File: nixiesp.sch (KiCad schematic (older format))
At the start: 50 parts, among them J1 Power 9-15V, J2 ESP8266, J3 Nixie PSU low, J4 CONN_01X02, Q1 BS107, Q2 BS107, Q3 BS107, Q4 BS107, U1 74HC595, U10 LM1117-3.3, U2 K155ID1, U3 K155ID1, U4 K155ID1, U5 74HC595, U6 K155ID1, U7 K155ID1, U8 74HC595

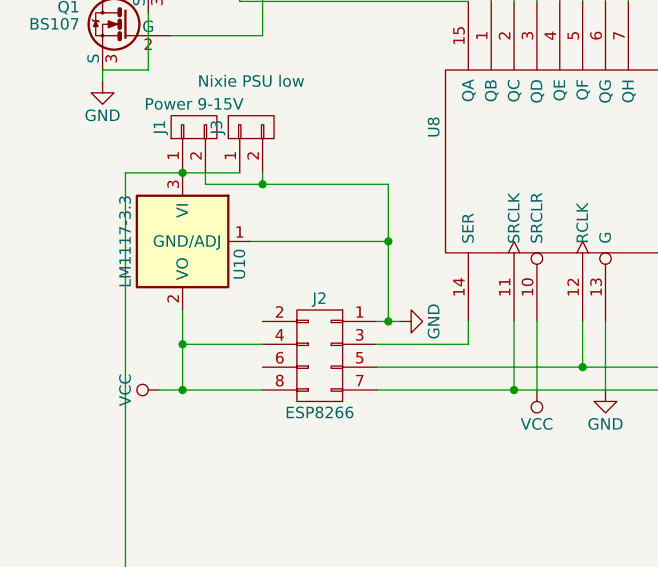
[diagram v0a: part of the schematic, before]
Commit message: Rotate tubes and other fixes
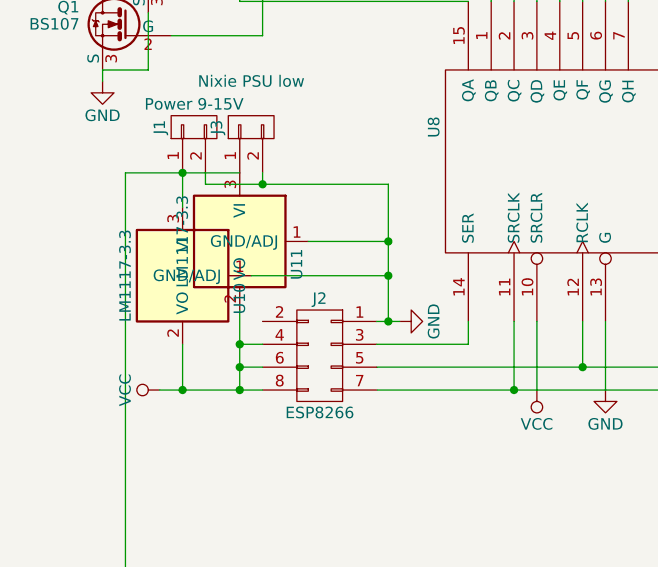
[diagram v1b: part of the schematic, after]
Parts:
- added U11: LM1117-3.3, TO_SOT_Packages_SMD:SOT-223, symbol LM1117-3.3
- U9: renamed from U?; value 74141-DIP -> K155ID1; footprint dip-sip:DIP-16 -> Housings_DIP:DIP-16_W7.62mm
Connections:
- wire segments 127 -> 131
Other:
- moved on the sheet: U10

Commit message: Hopefully final changes
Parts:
- removed D1, D10, D2, D3, D4, D9: LED, LEDs:LED_D5.0mm, symbol LED
- removed J3: Nixie PSU low, Pin_Headers:Pin_Header_Straight_1x02_Pitch2.54mm, symbol CONN_01X02
- removed J4: CONN_01X02, Pin_Headers:Pin_Header_Straight_1x02_Pitch2.54mm, symbol CONN_01X02
- removed R2, R3, R4, R5, R6: 330, Resistors_THT:R_Axial_DIN0204_L3.6mm_D1.6mm_P5.08mm_Horizontal, symbol R
- removed U10, U11: LM1117-3.3, TO_SOT_Packages_SMD:SOT-223, symbol LM1117-3.3
- added J10, J11, J12, J3, J4: CONN_01X06, Pin_Headers:Pin_Header_Angled_1x06_Pitch2.54mm, symbol CONN_01X06
- added J13: CONN_01X07, Pin_Headers:Pin_Header_Angled_1x07_Pitch2.54mm, symbol CONN_01X07
- added J14, J26: CONN_01X02, Pin_Headers:Pin_Header_Angled_1x02_Pitch2.54mm, symbol CONN_01X02
- added J15, J16, J17, J18, J19, J20, J21, J22, J23, J24, J25, J6, J7, J8: CONN_01X01, Connectors:1pin, symbol CONN_01X01
- added J27, J28, J29, J30, J5: CONN_01X06, Socket_Strips:Socket_Strip_Straight_1x06_Pitch2.54mm, symbol CONN_01X06
- added J31: CONN_01X07, Socket_Strips:Socket_Strip_Straight_1x07_Pitch2.54mm, symbol CONN_01X07
- added J32, J33: CONN_01X02, Socket_Strips:Socket_Strip_Straight_1x02_Pitch2.54mm, symbol CONN_01X02
- added J9: CONN_01X05, Socket_Strips:Socket_Strip_Straight_1x05_Pitch2.54mm, symbol CONN_01X05
- added U10: LM1117-5.0, TO_SOT_Packages_SMD:SOT-223, symbol LM1117-5.0
- added U11, U13, U14: 74HC595, Housings_DIP:DIP-16_W7.62mm, symbol 74HC595
- added U12: LM1117-3.3, TO_SOT_Packages_SMD:SOT-223, symbol LM1117-3.3
- J1: footprint Connectors:BARREL_JACK -> Connectors_Terminal_Blocks:TerminalBlock_Pheonix_PT-3.5mm_2pol
- Q1, Q2, Q3, Q4: footprint TO_SOT_Packages_THT:TO-92_Molded_Narrow -> TO_SOT_Packages_THT:TO-92_Inline_Wide
- R1: value 330 -> 2.2k; footprint Resistors_THT:R_Axial_DIN0204_L3.6mm_D1.6mm_P5.08mm_Horizontal -> Resistors_THT:R_Axial_DIN0207_L6.3mm_D2.5mm_P7.62mm_Horizontal
- R10, R11, R12, R13, R14, R15, R16, R7, R8, R9: footprint Resistors_THT:R_Axial_DIN0204_L3.6mm_D1.6mm_P5.08mm_Horizontal -> Resistors_THT:R_Axial_DIN0207_L6.3mm_D2.5mm_P7.62mm_Horizontal
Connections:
- net labels added: clock, data, latch
- wire segments 131 -> 230
- no-connect marks 2 -> 4
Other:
- moved on the sheet: J1, J2, N1, N10, N2, N3, N4, N5, N6, N7, N8, N9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
